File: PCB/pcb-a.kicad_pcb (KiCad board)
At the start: 2 copper layers, 116.3 x 50.4 mm, 38 parts, among them Q1 BC337, Q2 BC337, Q3 BC337, Q4 BC337, SW1 SW_DIP_x02, U1 MCP23008-xP, U4 ATmega16L-8P

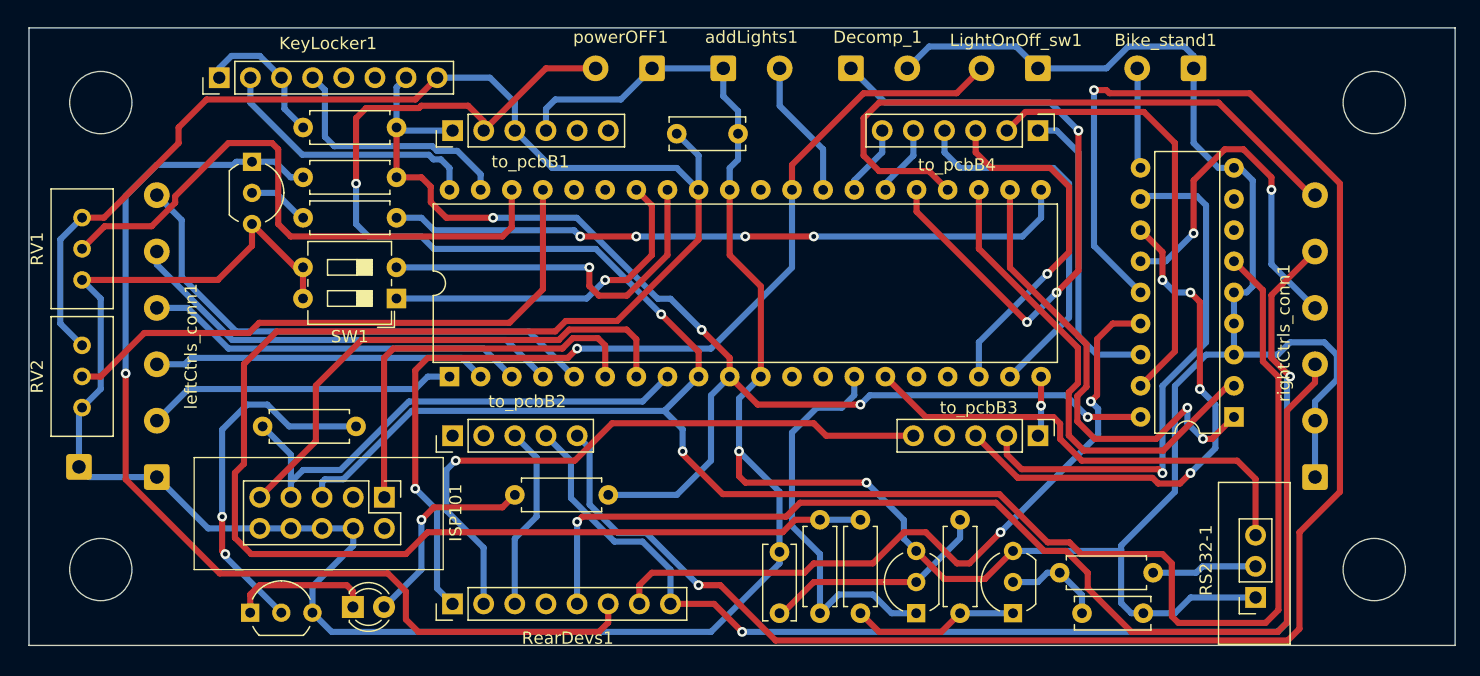
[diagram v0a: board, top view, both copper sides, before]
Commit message: fixes
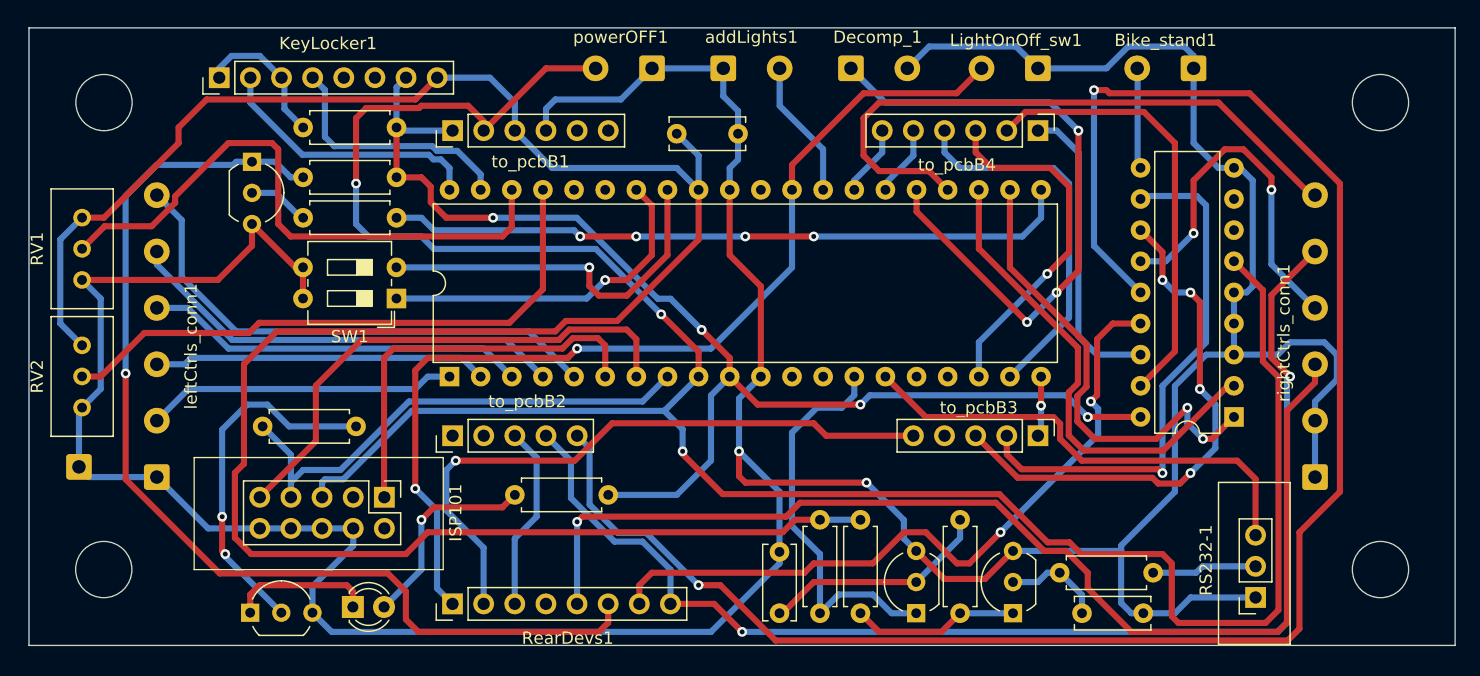
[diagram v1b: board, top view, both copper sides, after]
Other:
- outline, holes or cut-outs redrawn
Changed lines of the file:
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@@
   (gr_rect (start 196.604 93.106) (end 202.446 106.314) (layer "F.SilkS") (width 0.12) (fill none))
   (gr_rect (start 113.038 91.074) (end 133.358 100.218) (layer "F.SilkS") (width 0.1) (fill none))
-  (gr_circle (center 209.309589 62.112478) (end 211.849589 62.112478) (layer "Edge.Cuts") (width 0.05) (fill none))
-  (gr_circle (center 209.309589 100.212478) (end 211.849589 100.212478) (layer "Edge.Cuts") (width 0.05) (fill none))
-  (gr_circle (center 105.423589 100.212478) (end 107.963589 100.212478) (layer "Edge.Cuts") (width 0.05) (fill none))
-  (gr_circle (center 105.423589 62.118) (end 107.963589 62.118) (layer "Edge.Cuts") (width 0.05) (fill none))
+  (gr_circle (center 105.682866 62.118) (end 107.963522 61.869522) (layer "Edge.Cuts") (width 0.05) (fill none))
+  (gr_circle (center 209.817344 62.118) (end 212.098 61.869522) (layer "Edge.Cuts") (width 0.05) (fill none))
+  (gr_circle (center 209.817344 100.212478) (end 212.098 99.964) (layer "Edge.Cuts") (width 0.05) (fill none))
+  (gr_circle (center 105.663849 100.212478) (end 107.944505 99.964) (layer "Edge.Cuts") (width 0.05) (fill none))
   (gr_rect (start 99.565 56.022) (end 215.908 106.402) (layer "Edge.Cuts") (width 0.05) (fill none))
-  (gr_circle (center 105.672 100.212478) (end 111.514 100.466545) (layer "Margin") (width 0.1) (fill none))
-  (gr_circle (center 105.672 62.118) (end 111.514 62.372067) (layer "Margin") (width 0.1) (fill none))
-  (gr_circle (center 209.558 100.212478) (end 215.4 100.466545) (layer "Margin") (width 0.1) (fill none))
-  (gr_circle (center 209.558 62.112478) (end 215.4 62.366545) (layer "Margin") (width 0.1) (fill none))
+  (gr_circle (center 209.812 100.212478) (end 215.654 100.466545) (layer "Margin") (width 0.1) (fill none))
+  (gr_circle (center 105.658505 100.212478) (end 111.500505 100.466545) (layer "Margin") (width 0.1) (fill none))
+  (gr_circle (center 105.677522 62.118) (end 111.519522 62.372067) (layer "Margin") (width 0.1) (fill none))
+  (gr_circle (center 209.812 62.118) (end 215.654 62.372067) (layer "Margin") (width 0.1) (fill none))
   (dimension (type aligned) (layer "B.Mask")
-    (pts (xy 99.576 55.68) (xy 216.427 55.68))
+    (pts (xy 99.565 56.022) (xy 215.908 56.022))
     (height -4.738)
-    (gr_text "116,8510 mm" (at 158.0015 49.792) (layer "B.Mask")
+    (gr_text "116,3430 mm" (at 157.7365 50.134) (layer "B.Mask")
       (effects (font (size 1 1) (thickness 0.15)))
     )
@@
   )
   (dimension (type aligned) (layer "B.Mask")
-    (pts (xy 105.423589 62.118) (xy 105.423589 100.212478))
+    (pts (xy 105.682866 62.118) (xy 105.663849 100.212478))
     (height 9.657589)
-    (gr_text "38,0945 mm" (at 94.616 81.165239 90) (layer "B.Mask")
+    (gr_text "38,0945 mm" (at 94.86577 81.159844 89.9713991) (layer "B.Mask")
       (effects (font (size 1 1) (thickness 0.15)))
     )
@@
   )
   (dimension (type aligned) (layer "B.Mask")
-    (pts (xy 105.423589 100.212478) (xy 209.309589 100.212478))
+    (pts (xy 105.658505 100.212478) (xy 209.812 100.212478))
     (height 10.927522)
-    (gr_text "103,8860 mm" (at 157.366589 109.99) (layer "B.Mask")
+    (gr_text "104,1535 mm" (at 157.735252 109.99) (layer "B.Mask")
       (effects (font (size 1 1) (thickness 0.15)))
     )
@@
   (segment (start 117.61 103.732) (end 117.61 102.25) (width 0.5) (layer "F.Cu") (net 73))
   (segment (start 125.484 101.488) (end 125.987 101.991) (width 0.5) (layer "F.Cu") (net 73))
-  (group "" (id 01a48bd9-2a0e-4b43-82a9-cdb8d78936d6)
+  (group "" (id 1191cbb4-e868-45f0-9b39-0c9024056cfc)
     (members
-      05553d34-2925-4bdc-8bab-f9f5b3c55f82
-      98c1bbca-1fff-4140-9564-036468572850
-    )
-  )
-  (group "" (id 253c07d0-8b56-443c-8c68-2271fb73760d)
+      1ea9ef13-f563-41d1-a8f6-1e2cb00ccbf7
+      9438a5aa-eef2-4593-ab90-e2163a57d33e
+    )
+  )
+  (group "" (id 238341a2-c60a-4837-b744-5691eaa33d93)
+    (members
+      3010c1c4-469c-4354-abc8-53d22652e3ed
+      c45d402f-1a26-4fe2-8344-1050baa32279
+    )
+  )
+  (group "" (id 9d6b8b74-bb01-4229-a181-a39289eb290b)
     (members
       198ffc1c-39e1-4c4c-8a2d-9dd88408dbde
@@
     )
   )
-  (group "" (id 61a310f2-1cb2-413c-8545-ec5ad506d193)
+  (group "" (id dbfaaa01-c9ae-441e-87c0-ab444ec25e89)
     (members
-      14dd9be3-aed6-412b-97ca-53051d9353e5
-      d13d56c9-9469-4be9-b6a0-277f87dc44ae
-    )
-  )
-  (group "" (id d2ff0935-d21d-40ba-8411-cf09b2b1f453)
-    (members
-      0f17db16-33e6-4476-b6db-e9f8db459e64
-      c424aa93-48f7-4c7a-98ff-3443ed3fcc41
-    )
-  )
+      35c22e0c-a422-413e-b740-b398cd6d7ad2
+      db7f76ad-4333-4102-9a41-cba291edbf3f
+    )
+  )
